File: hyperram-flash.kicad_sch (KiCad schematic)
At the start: 17 parts, among them U1 IS66WVH16M8DBLL-100B1LI, U3 S25FL128SAGNFI000

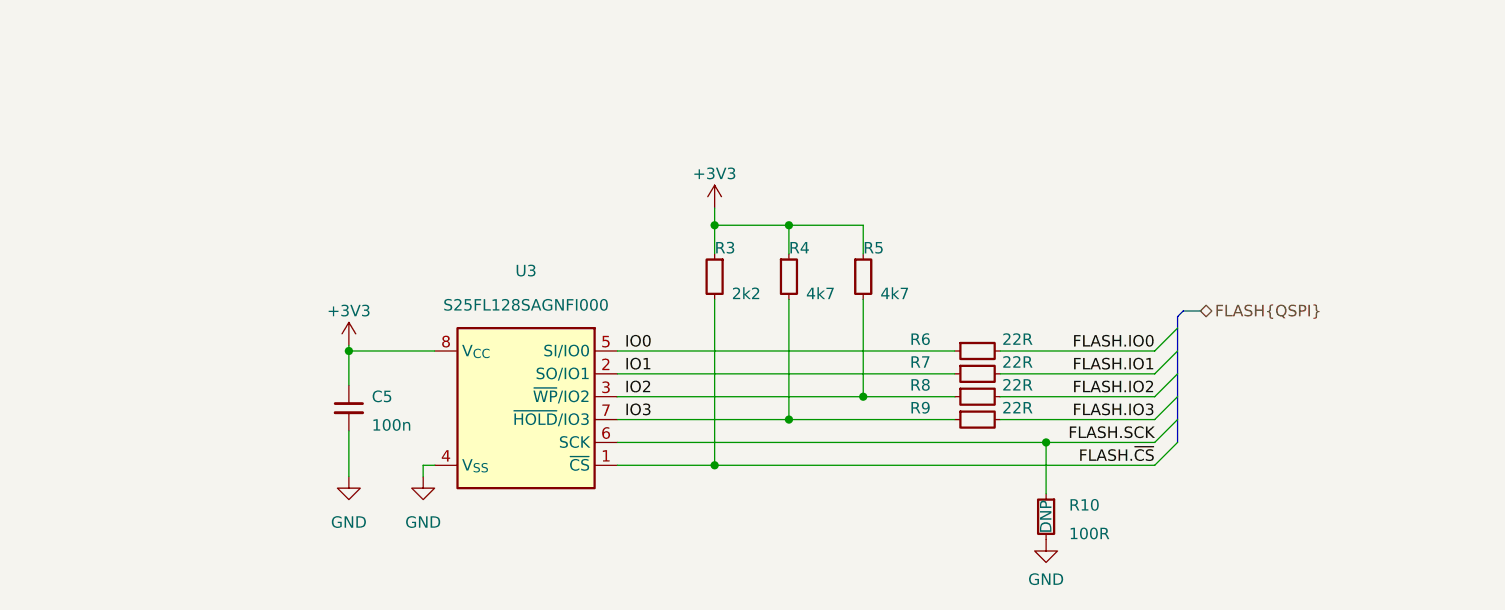
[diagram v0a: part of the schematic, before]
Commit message: Finish schematic cleanup
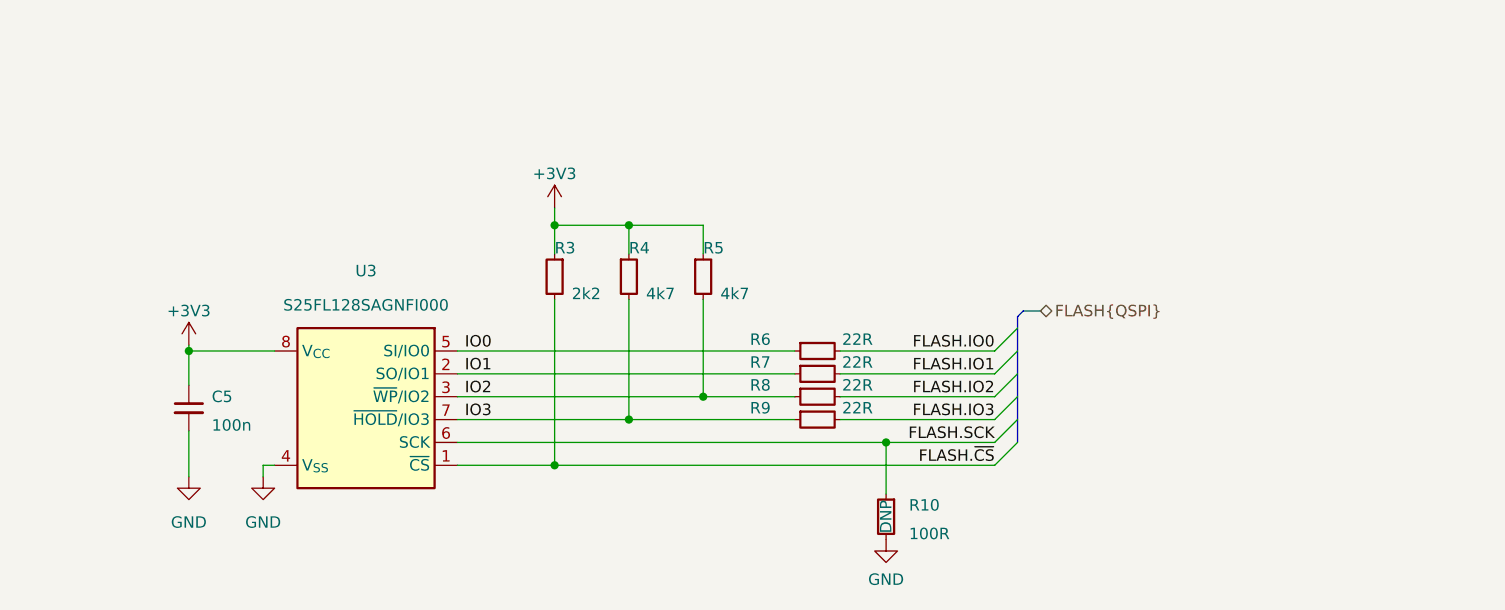
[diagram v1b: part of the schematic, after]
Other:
- moved on the sheet: C5, R10, R3, R4, R5, R6, R7, R8, R9, U3
